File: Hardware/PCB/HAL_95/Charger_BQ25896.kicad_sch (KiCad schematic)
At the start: 34 parts, among them J9 Conn_01x02, SW3 431183015816, U3 XC6206P332MR, U5 BQ25896RTW

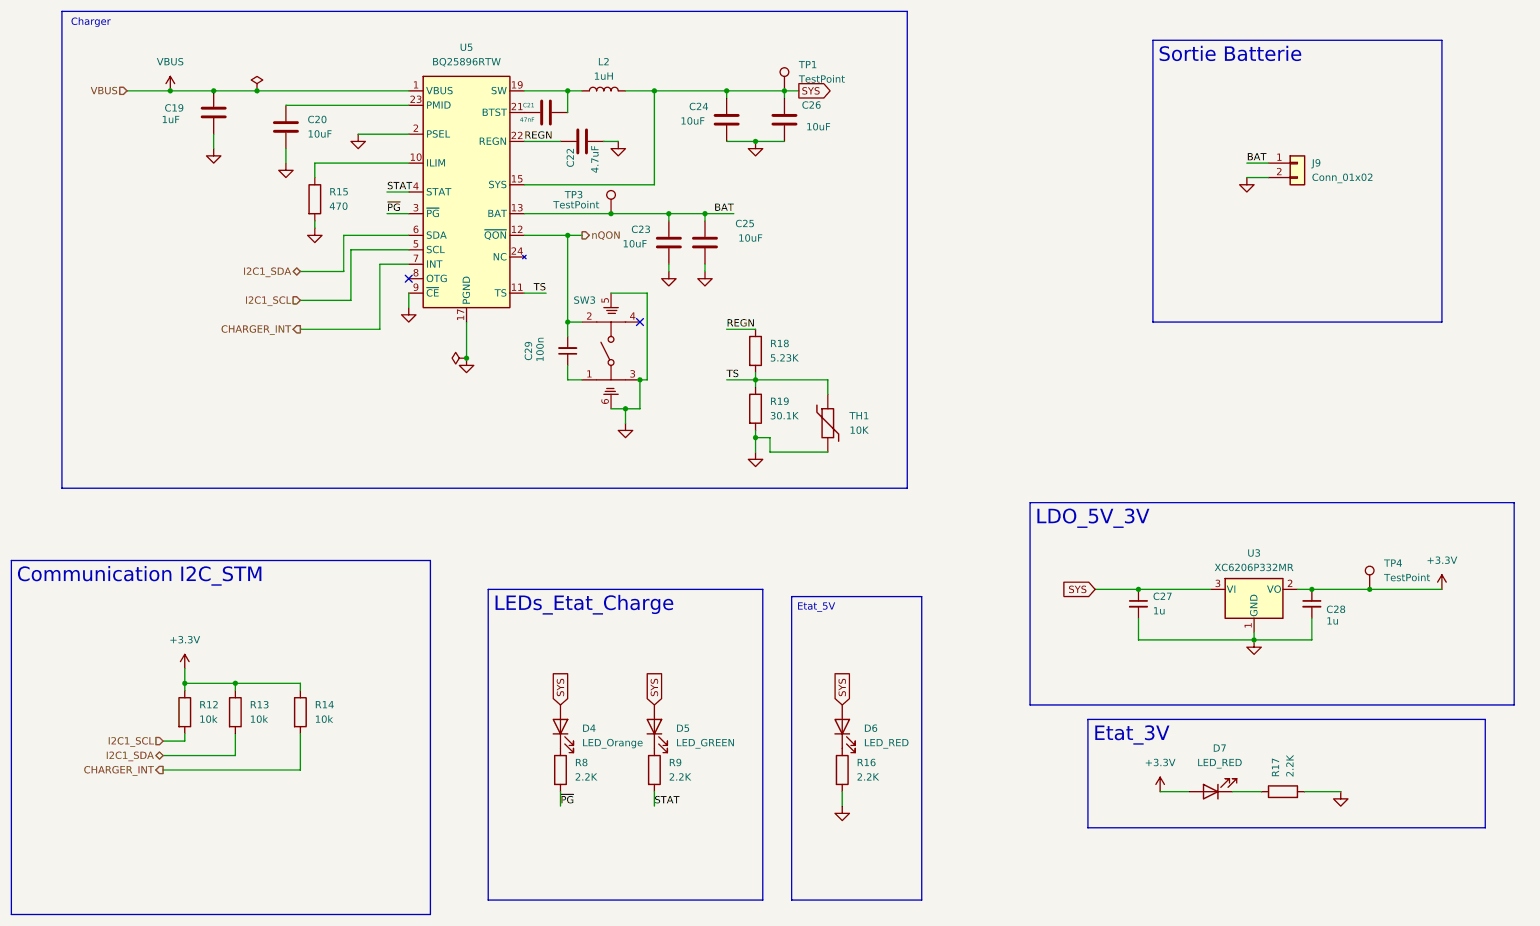
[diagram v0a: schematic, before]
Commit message: finished schematic
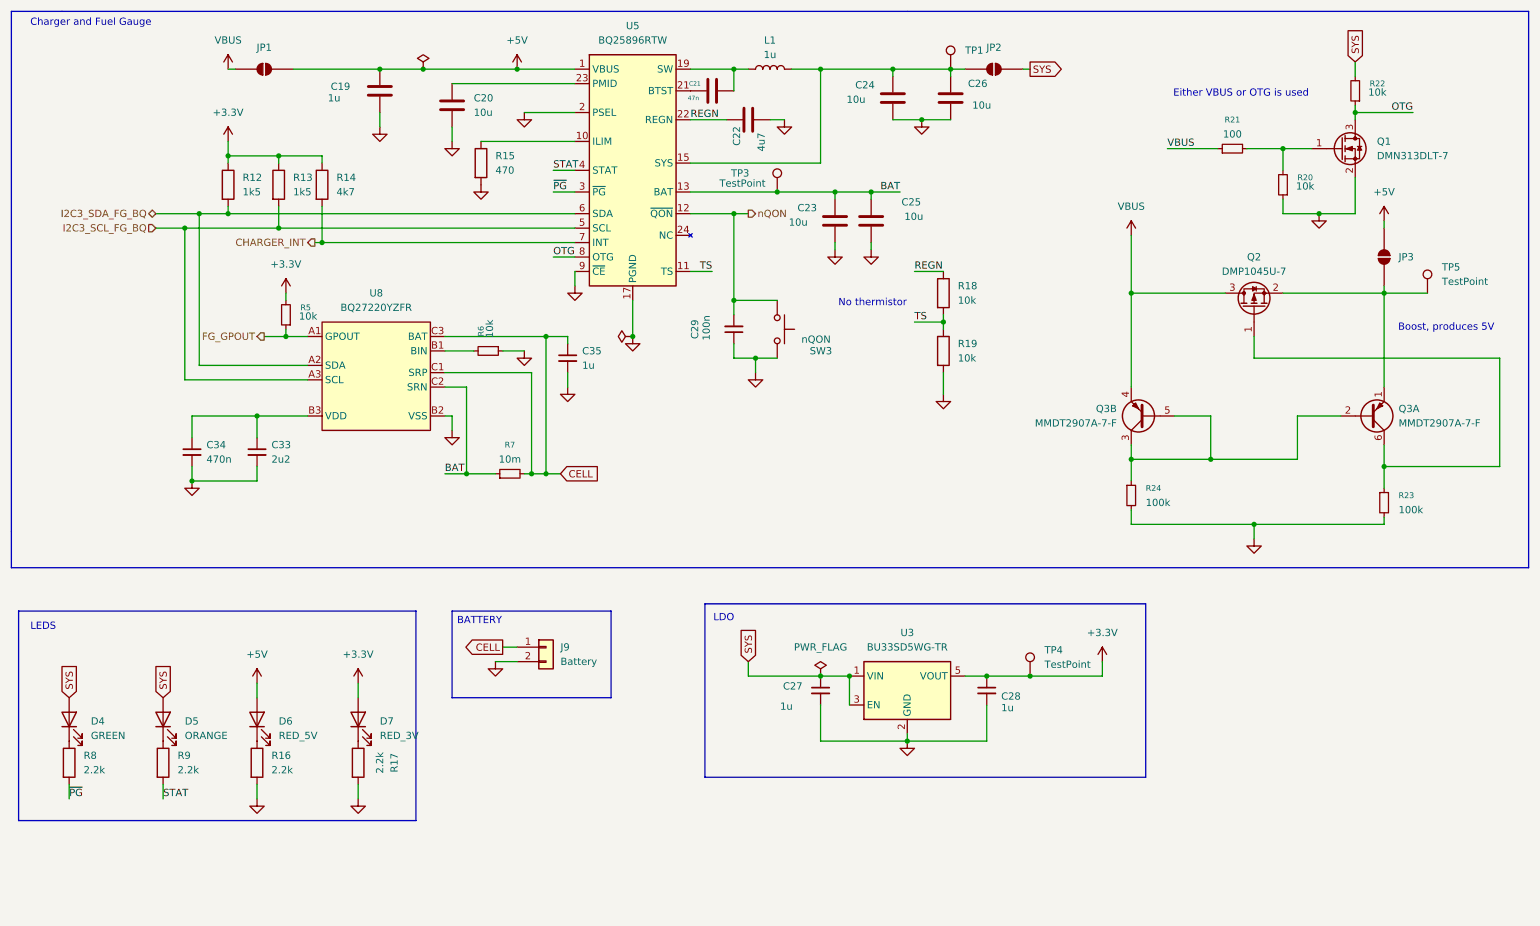
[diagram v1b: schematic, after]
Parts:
- removed SW3: 431183015816, Switch_SMD_Wurth:SW_Wurth_WS-TASV_431183015816, symbol Switch_Wurth_WS-TASV:431183015816
- removed TH1: 10K, Resistor_SMD:R_0603_1608Metric, symbol Device:Thermistor
- removed U3: XC6206P332MR, Package_TO_SOT_SMD:SOT-23-3, symbol Regulator_Linear:XC6206PxxxMR
- added C33: 2u2, Capacitor_SMD:C_0402_1005Metric, symbol Device:C_Small
- added C34: 470n, Capacitor_SMD:C_0402_1005Metric, symbol Device:C_Small
- added C35: 1u, Capacitor_SMD:C_0402_1005Metric, symbol Device:C_Small
- added JP1, JP2, JP3: SolderJumper_2_Open, symbol Jumper:SolderJumper_2_Open
- added Q1: DMN313DLT-7, Package_TO_SOT_SMD:SOT-523, symbol Transistor_FET:DMN3150L
- added Q2: DMP1045U-7, Package_TO_SOT_SMD:SOT-23, symbol Transistor_FET:DMP3099L
- added Q3: MMDT2907A-7-F, Package_TO_SOT_SMD:SOT-363_SC-70-6, symbol Transistor_BJT:MMDT3906
- added R20, R22, R5, R6: 10k, Resistor_SMD:R_0402_1005Metric, symbol Device:R_Small
- added R21: 100, Resistor_SMD:R_0402_1005Metric, symbol Device:R_Small
- added R23, R24: 100k, Resistor_SMD:R_0402_1005Metric, symbol Device:R_Small
- added R7: 10m, Resistor_SMD:R_2512_6332Metric, symbol Device:R_Small
- added SW3: nQON, Button_Switch_SMD:SW_Push_1P1T_NO_CK_KMR2, symbol Switch:SW_Push
- added TP5: TestPoint, TestPoint:TestPoint_Pad_D2.0mm, symbol Connector:TestPoint
- added U3: BU33SD5WG-TR, Package_TO_SOT_SMD:SOT-23-5, symbol Regulator_Linear:MIC5365-3.3YD5
- added U8: BQ27220YZFR, Package_BGA:BGA-9_1.6x1.6mm_Layout3x3_P0.5mm, symbol power_lib:BQ27220YZFR
- C19: value 1uF -> 1u
- C20, C23, C24, C25, C26: value 10uF -> 10u; footprint Capacitor_SMD:C_0402_1005Metric -> Capacitor_SMD:C_0603_1608Metric; JLCPCB Part # C15525 -> C70225
- C21: value 47nF -> 47n; JLCPCB Part # C384812 -> C82219
- C22: value 4.7uF -> 4u7
- C27, C28: JLCPCB Part # C52923 -> C29266
- D4: value LED_Orange -> GREEN; JLCPCB Part # C84269 -> C99289
- D5: value LED_GREEN -> ORANGE; footprint Button_Switch_THT:SW_NKK_GW12LJP -> LED_SMD:LED_0603_1608Metric; JLCPCB Part # C99289 -> C84269
- D6: value LED_RED -> RED_5V; footprint Button_Switch_THT:SW_NKK_GW12LJP -> LED_SMD:LED_0603_1608Metric
- D7: value LED_RED -> RED_3V; footprint Button_Switch_THT:SW_NKK_GW12LJP -> LED_SMD:LED_0603_1608Metric
- J9: value Conn_01x02 -> Battery
- L1: renamed from L2; value 1uH -> 1u; footprint Inductor_SMD:L_0201_0603Metric -> Inductor_SMD:L_0402_1005Metric; JLCPCB Part # C22037 -> C531284
- R12, R13: value 10k -> 1k5; JLCPCB Part # C25744 -> C25867
- R14: value 10k -> 4k7; JLCPCB Part # C25744 -> C25900
- R16, R17, R8, R9: value 2.2K -> 2.2k; JLCPCB Part # C25744 -> C25879
- R18: value 5.23K -> 10k; JLCPCB Part # C25905 -> C25531
- R19: value 30.1K -> 10k; JLCPCB Part # C25779 -> C25531
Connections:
- net +3.3V: now also R5.2, U3.5 (VOUT)
- net BAT: now also R7.1, U8.C2 (SRN); no longer J9.1 (Pin_1)
- net GND: now also C29.1, C33.2, C34.2, C35.2, Q1.2 (S), R20.1, R23.2, R24.2, R6.1, SW3.2, U3.2 (GND), U8.B2 (VSS)
- net SYS: now also JP2.2 (B), R22.2, U3.1 (VIN), U3.3 (EN); no longer C24.1, C26.1, D6.2 (A), L1.2, TP1.1, U5.15 (SYS), U5.16 (SYS)
- net VBUS: now also JP1.1 (A), Q2.3 (D), Q3.4 (E2), R21.1; no longer C19.1, U5.1 (VBUS)
- net nQON: now also SW3.1
- net OTG: now reaches U5.8 (OTG)
- net OTG: now also Q1.3 (D), R22.1
- net I2C1_SCL renamed I2C3_SCL_FG_BQ
- net I2C3_SCL_FG_BQ: now also R13.2, U8.A3 (SCL); no longer R12.2
- net I2C1_SDA renamed I2C3_SDA_FG_BQ
- net I2C3_SDA_FG_BQ: now also R12.2, U8.A2 (SDA); no longer R13.2
- new net: Q3.2 (B1), Q3.3 (C2), Q3.5 (B2), R24.1
- new net: C24.1, C26.1, JP2.1 (A), L1.2, TP1.1, U5.15 (SYS), U5.16 (SYS)
- new net: JP3.1 (A), Q2.2 (S), Q3.1 (E1), TP5.1
- new net: Q2.1 (G), Q3.6 (C1), R23.1
- new net: R6.2, U8.B1 (BIN)
- new net: C33.1, C34.1, U8.B3 (VDD)
- new net: Q1.1 (G), R20.2, R21.2
- new net +5V: C19.1, D6.2 (A), JP1.2 (B), JP3.2 (B), U5.1 (VBUS)
- new net CELL: C35.1, J9.1 (Pin_1), R7.2, U8.C1 (SRP), U8.C3 (BAT)
- new net FG_GPOUT: R5.1, U8.A1 (GPOUT)
- no-connect marks 2 -> 0
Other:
- note added: "BATTERY"
- note added: "Boost, produces 5V"
- note added: "Charger and Fuel Gauge"
- note added: "Either VBUS or OTG is used"
- note added: "LDO"
- note added: "LEDS"
- note added: "No thermistor"
- note removed: "Charger"
- moved on the sheet: C19, C20, C21, C22, C23, C24, C25, C26, C28, C29, D4, D5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
